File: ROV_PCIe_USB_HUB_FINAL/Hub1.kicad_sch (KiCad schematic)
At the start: 22 parts, among them J4 SM04B-SRSS-TB, J5 SM04B-SRSS-TB, U3 USB2422/MJ, U4 TPS2051CDBV, U5 TPS2051CDBV, Y2 ECS-240-8-37B-CKY-TR

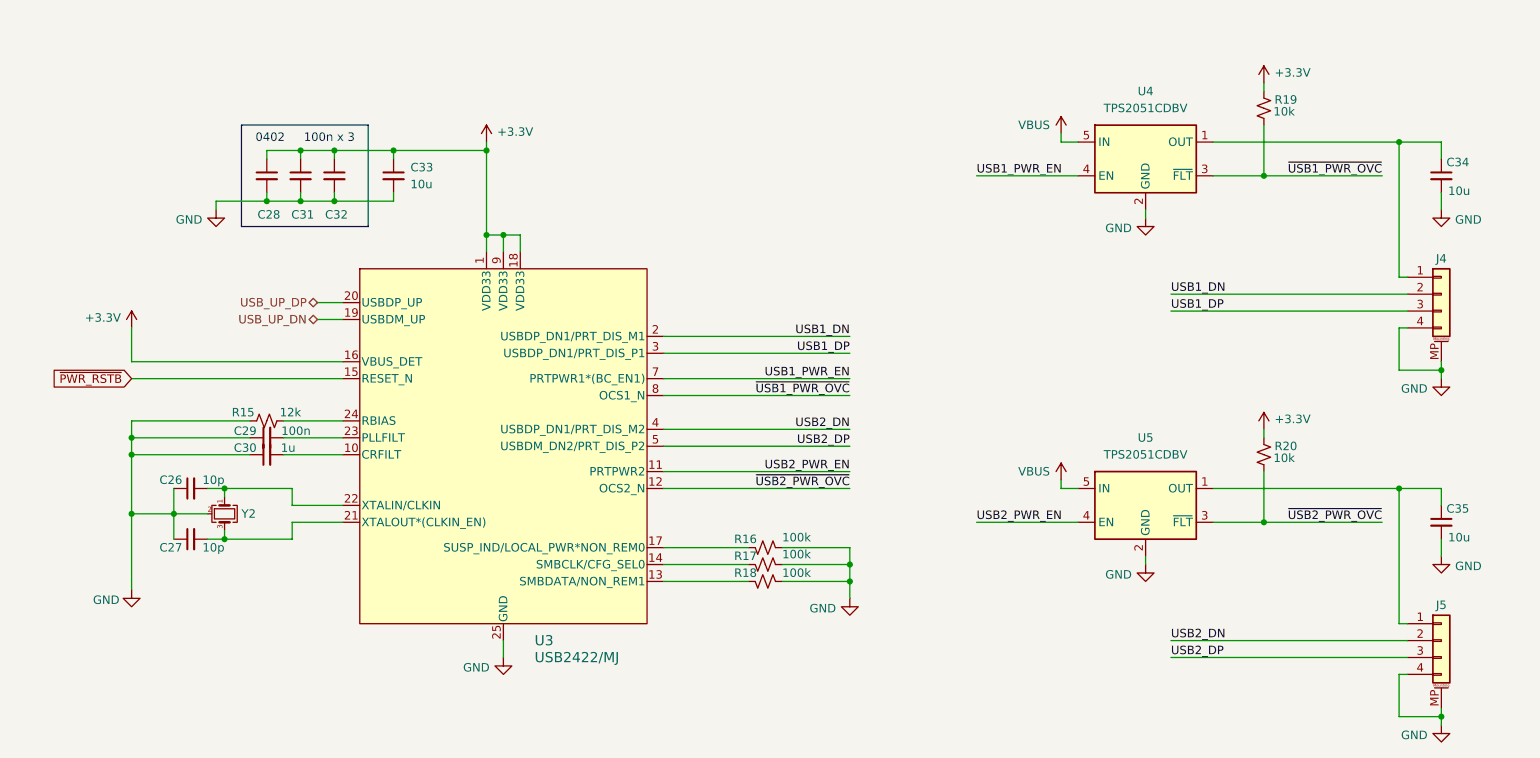
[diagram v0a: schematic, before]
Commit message: changes
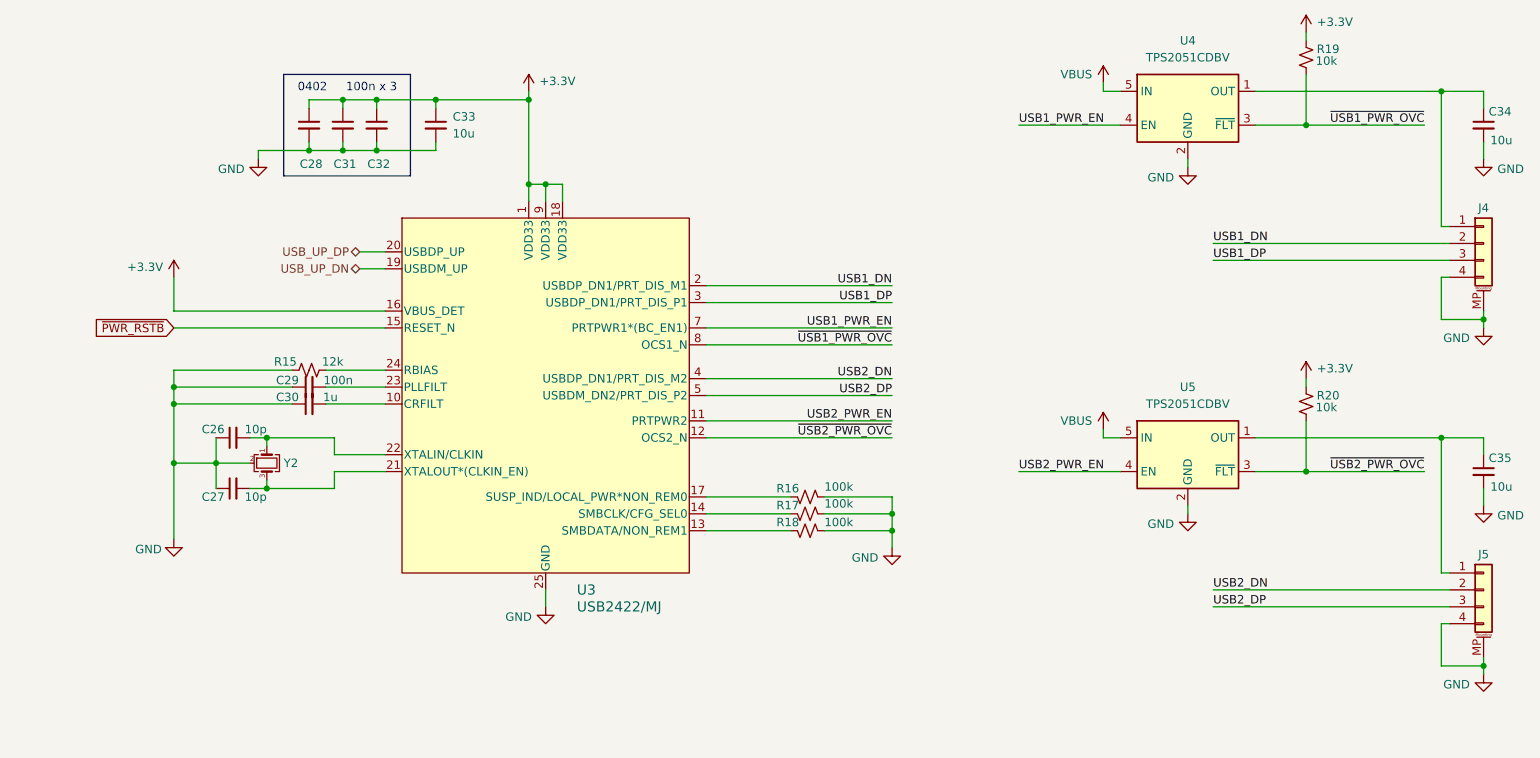
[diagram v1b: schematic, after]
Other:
- moved on the sheet: C26, C27, C28, C29, C30, C31, C33, C34, C35, J4, J5, R15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
